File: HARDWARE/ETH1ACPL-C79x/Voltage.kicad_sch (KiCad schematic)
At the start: 55 parts, among them J501 1710072, U501 DG412LEDQ, U502 DG419LEDY, U503 TBA 1-0511HI, U504 ACPL-C79B, U505 OPA2340UA

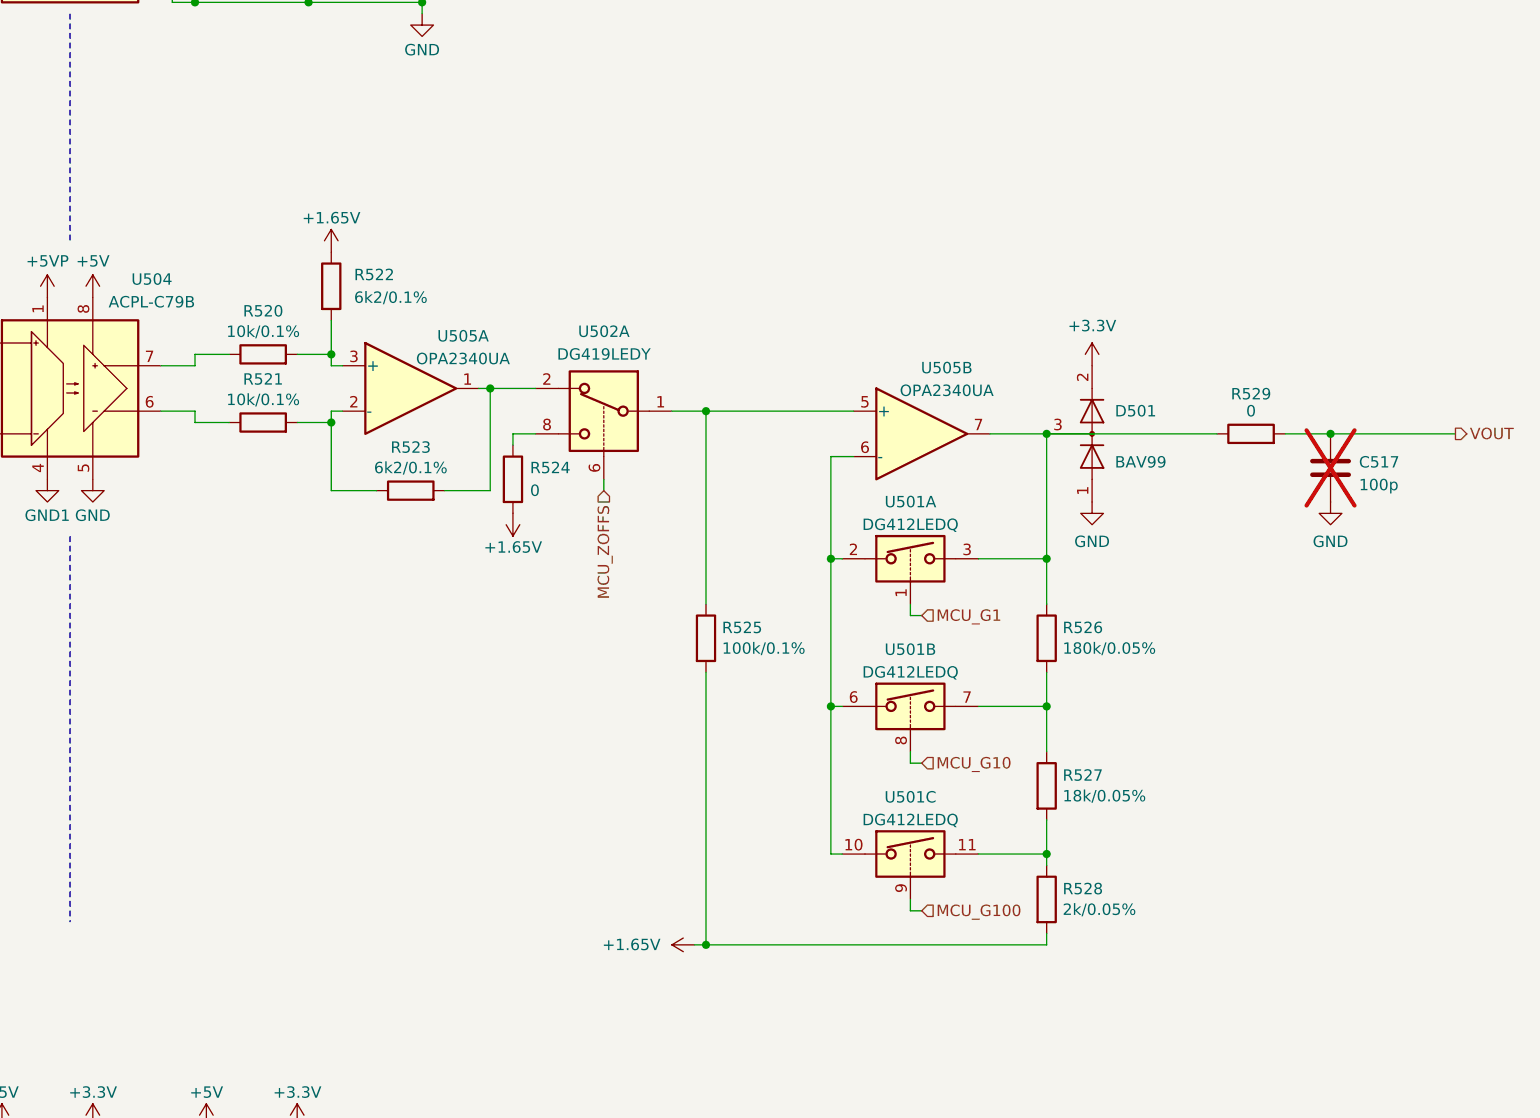
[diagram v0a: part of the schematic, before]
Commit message: Hardware design
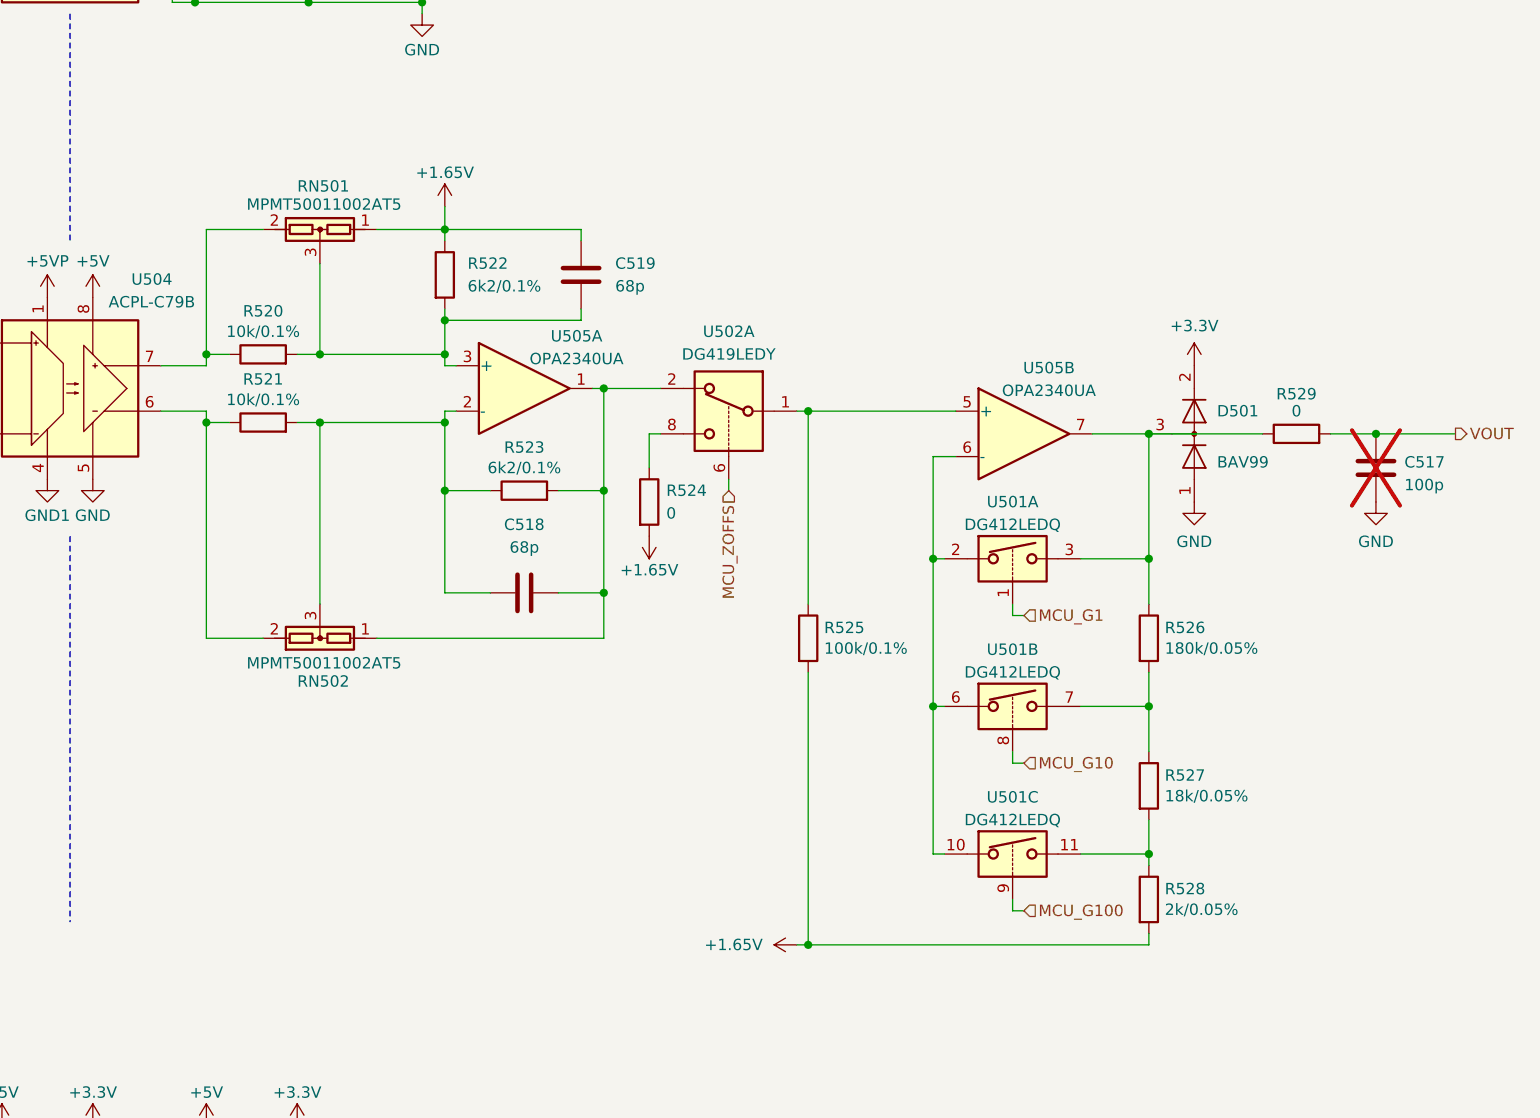
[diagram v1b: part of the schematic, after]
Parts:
- added C518, C519: 68p, Capacitor_SMD:C_0603_1608Metric_Pad1.08x0.95mm_HandSolder, symbol Device:C
- added RN501, RN502: MPMT50011002AT5, Package_TO_SOT_SMD:SOT-23, symbol Device:VoltageDivider_CenterPin3
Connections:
- net +1.65V: now also C519.2, RN501.1
- net at R520.2, R522.2, U505.3 (+): now also C519.1, RN501.3
- net at R521.2, R523.1, U505.2 (-): now also C518.1, RN502.3
- net at R523.2, U502.2, U505.1: now also C518.2, RN502.1
- net at R520.1, U504.7 (OUT+): now also RN501.2
- net at R521.1, U504.6 (OUT-): now also RN502.2
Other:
- moved on the sheet: C517, D501, R522, R523, R524, R525, R526, R527, R528, R529, U501A, U501B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
